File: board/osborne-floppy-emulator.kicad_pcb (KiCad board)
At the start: 2 copper layers, 61.6 x 54 mm, 82 parts, among them J1 Connector Out, J2 USB_A, J3 SWD Connector, J4 Connector In, Q1 BC557, Q2 BC547, Q3 T2N7002BK, Q4 BC847C, Q5 BC847C, Q6 BC847C, Q7 BC847C, Q8 BC847C, Q9 BC847C, U1 W25Q16JVSSIM, U2 RP2040, U3 TL494

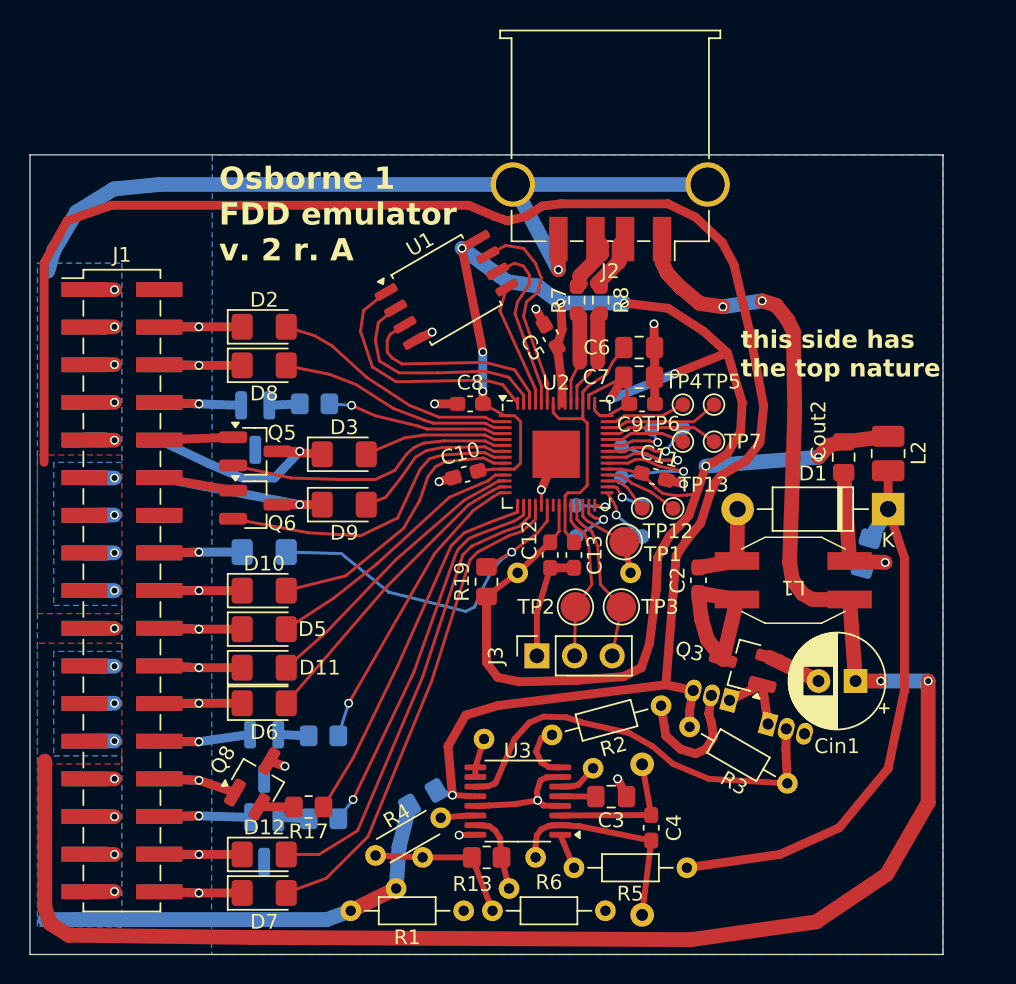
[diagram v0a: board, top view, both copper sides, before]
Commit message: shrink board slightly
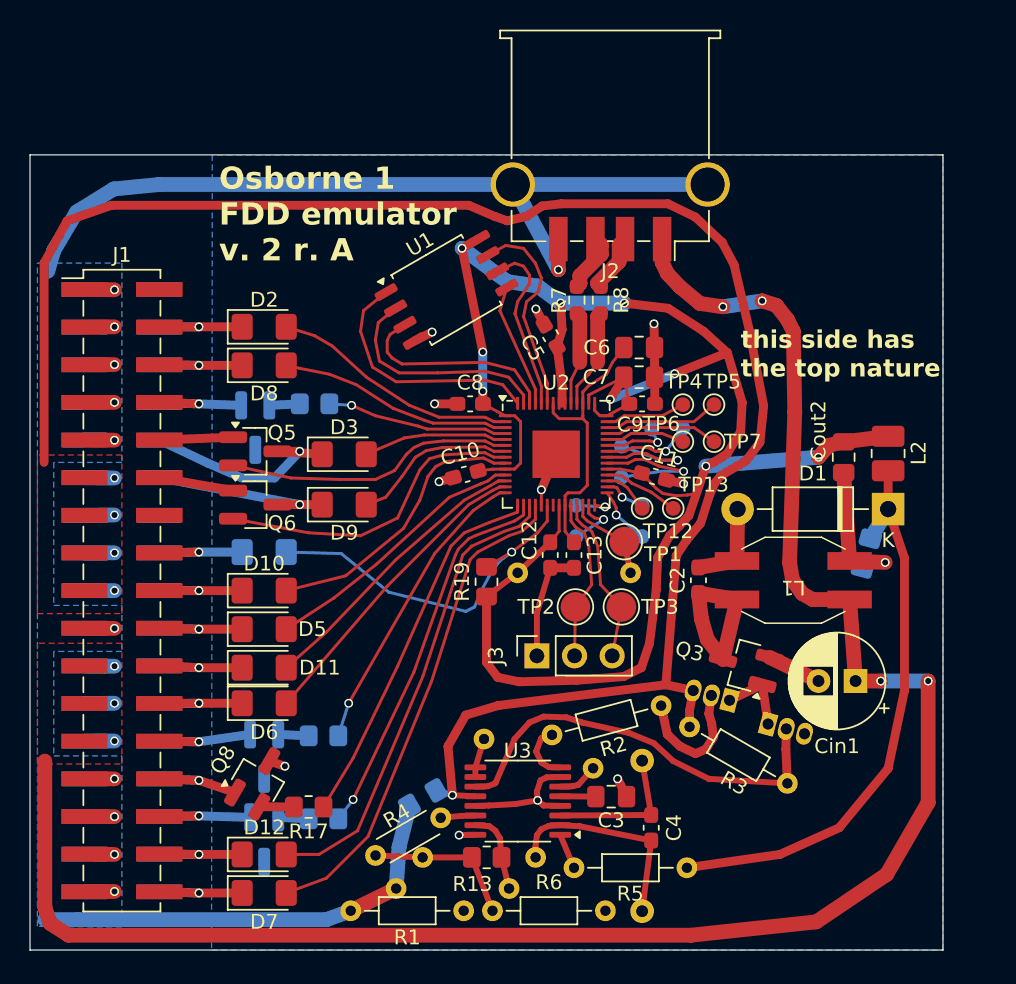
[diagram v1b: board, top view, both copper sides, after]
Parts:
- moved R11 0.25 mm to (131.7, 93.9)
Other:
- board size 61.6 x 54 mm -> 61.6 x 53.7 mm
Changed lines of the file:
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@@
 	(footprint "Resistor_THT:R_Axial_DIN0207_L6.3mm_D2.5mm_P10.16mm_Horizontal"
 		(layer "B.Cu")
-		(at 131.7 94.12 -90)
+		(at 131.7 93.87 -90)
 		(descr "Resistor, Axial_DIN0207 series, Axial, Horizontal, pin pitch=10.16mm, 0.25W = 1/4W, length*diameter=6.3*2.5mm^2, http://cdn-reichelt.de/documents/datenblatt/B400/1_4W%23YAG.pdf")
 		(tags "Resistor Axial_DIN0207 series Axial Horizontal pin pitch 10.16mm 0.25W = 1/4W length 6.3mm diameter 2.5mm")
@@
 	(gr_rect
 		(start 90.4 53)
-		(end 152 106.95)
+		(end 152 106.65)
 		(stroke
 			(width 0.05)
@@
 	)
 	(segment
-		(start 132.3125 99.2625)
-		(end 131.7 104.279999)
+		(start 126.175 98.225)
+		(end 125.4 98.275)
 		(width 0.4)
 		(layer "F.Cu")
@@
 	)
 	(segment
-		(start 126.175 98.225)
-		(end 125.4 98.275)
+		(start 127.5 98.3)
+		(end 132.3125 99.2625)
 		(width 0.4)
 		(layer "F.Cu")
@@
 	)
 	(segment
-		(start 127.5 98.3)
-		(end 132.3125 99.2625)
+		(start 132.3125 99.2625)
+		(end 131.7 104.03)
 		(width 0.4)
 		(layer "F.Cu")
@@
 	(segment
 		(start 132.3125 97.5375)
-		(end 131.7 94.12)
+		(end 131.7 93.87)
 		(width 0.4)
 		(layer "F.Cu")
@@
 	)
 	(segment
-		(start 91.4 103.75)
-		(end 91.4 93.9)
-		(width 1)
-		(layer "F.Cu")
-		(net 11)
-	)
-	(segment
-		(start 148.2 101.55)
-		(end 143.45 104.75)
+		(start 91.75 104.85)
+		(end 91.4 103.75)
 		(width 1)
 		(layer "F.Cu")
@@
 	)
 	(segment
-		(start 143.2 83)
-		(end 145.700001 83)
+		(start 91.4 103.75)
+		(end 91.4 93.9)
 		(width 1)
 		(layer "F.Cu")
@@
 	)
 	(segment
-		(start 151 88.5)
-		(end 151 96.7)
+		(start 143.2 83)
+		(end 145.700001 83)
 		(width 1)
 		(layer "F.Cu")
@@
 	)
 	(segment
-		(start 146.099999 88.5)
-		(end 147.8 88.5)
+		(start 151 96.7)
+		(end 148.2 101.55)
 		(width 1)
 		(layer "F.Cu")
@@
 	)
 	(segment
-		(start 91.75 104.85)
-		(end 91.4 103.75)
+		(start 148.2 101.55)
+		(end 143.45 104.75)
 		(width 1)
 		(layer "F.Cu")
@@
 	)
 	(segment
-		(start 135 105.95)
-		(end 105.4 105.8)
+		(start 146.099999 88.5)
+		(end 147.8 88.5)
 		(width 1)
 		(layer "F.Cu")
@@
 	)
 	(segment
-		(start 105.4 105.8)
-		(end 93 105.65)
+		(start 142.5 82.6)
+		(end 143.2 83)
 		(width 1)
 		(layer "F.Cu")
@@
 	)
 	(segment
-		(start 151 96.7)
-		(end 148.2 101.55)
+		(start 139.8 62.85)
+		(end 140.75 63.15)
 		(width 1)
 		(layer "F.Cu")
@@
 	)
 	(segment
-		(start 143.45 104.75)
-		(end 135 105.95)
+		(start 137.15 63.25)
+		(end 135.6 63.026923)
 		(width 1)
 		(layer "F.Cu")
@@
 	)
 	(segment
-		(start 142.5 82.6)
-		(end 143.2 83)
+		(start 141.9 64.9)
+		(end 142 70.35)
 		(width 1)
 		(layer "F.Cu")
@@
 	)
 	(segment
-		(start 93 105.65)
-		(end 91.75 104.85)
+		(start 141.5 64.1)
+		(end 141.9 64.9)
 		(width 1)
 		(layer "F.Cu")
@@
 	)
 	(segment
-		(start 139.8 62.85)
-		(end 140.75 63.15)
+		(start 93 105.65)
+		(end 91.75 104.85)
 		(width 1)
 		(layer "F.Cu")
@@
 	)
 	(segment
-		(start 137.15 63.25)
-		(end 135.6 63.026923)
+		(start 135 105.65)
+		(end 93 105.65)
 		(width 1)
 		(layer "F.Cu")
@@
 	)
 	(segment
-		(start 141.9 64.9)
-		(end 142 70.35)
+		(start 143.45 104.75)
+		(end 135 105.65)
 		(width 1)
 		(layer "F.Cu")
@@
 	)
 	(segment
-		(start 141.5 64.1)
-		(end 141.9 64.9)
+		(start 135.6 63.026923)
+		(end 134.25 61.9)
 		(width 1)
 		(layer "F.Cu")
@@
 	)
 	(segment
-		(start 135.6 63.026923)
-		(end 134.25 61.9)
+		(start 151 88.5)
+		(end 151 96.7)
 		(width 1)
 		(layer "F.Cu")
@@
 	)
 	(segment
-		(start 125.05 90.9)
-		(end 126.6 90.95)
-		(width 0.4)
-		(layer "F.Cu")
-		(net 50)
-	)
-	(segment
-		(start 126.6 90.95)
-		(end 127.65 91.3)
+		(start 121.3 95.6)
+		(end 121.8 95.4)
 		(width 0.4)
 		(layer "F.Cu")
@@
 	)
 	(segment
-		(start 136.2 95.1)
-		(end 141.499556 95.405)
+		(start 130.8 92)
+		(end 132.5 92.7)
 		(width 0.4)
 		(layer "F.Cu")
@@
 	)
 	(segment
-		(start 127.65 91.3)
-		(end 130.8 92)
+		(start 125.05 90.9)
+		(end 126.6 90.95)
 		(width 0.4)
 		(layer "F.Cu")
@@
 	)
 	(segment
-		(start 124.1 91.3)
-		(end 125.05 90.9)
+		(start 132.5 92.7)
+		(end 133.8 93.9)
 		(width 0.4)
 		(layer "F.Cu")
@@
 	)
 	(segment
-		(start 120.45 95.625)
-		(end 121.3 95.6)
+		(start 127.65 91.3)
+		(end 130.8 92)
 		(width 0.4)
 		(layer "F.Cu")
@@
 	)
 	(segment
-		(start 121.8 95.4)
-		(end 122.4 94)
+		(start 120.45 95.625)
+		(end 121.3 95.6)
 		(width 0.4)
 		(layer "F.Cu")
@@
 	)
 	(segment
-		(start 132.4 92.9)
-		(end 133.8 94.1)
+		(start 123.1 92.4)
+		(end 124.1 91.3)
 		(width 0.4)
 		(layer "F.Cu")
@@
 	)
 	(segment
-		(start 122.4 94)
-		(end 123.1 92.4)
+		(start 126.6 90.95)
+		(end 127.65 91.3)
 		(width 0.4)
 		(layer "F.Cu")
@@
 	)
 	(segment
-		(start 133.8 94.1)
-		(end 136.2 95.1)
+		(start 136.2 95.1)
+		(end 141.499556 95.405)
 		(width 0.4)
 		(layer "F.Cu")
@@
 	)
 	(segment
-		(start 121.3 95.6)
-		(end 121.8 95.4)
+		(start 121.8 95.4)
+		(end 122.4 94)
 		(width 0.4)
 		(layer "F.Cu")
@@
 	)
 	(segment
-		(start 130.8 92)
-		(end 132.4 92.9)
+		(start 122.4 94)
+		(end 123.1 92.4)
 		(width 0.4)
 		(layer "F.Cu")
@@
 	)
 	(segment
-		(start 123.1 92.4)
-		(end 124.1 91.3)
+		(start 133.8 93.9)
+		(end 136.2 95.1)
 		(width 0.4)
 		(layer "F.Cu")
@@
 	)
 	(segment
-		(start 136.4 91.4)
-		(end 136.2 90.7)
+		(start 124.1 91.3)
+		(end 125.05 90.9)
+		(width 0.4)
+		(layer "F.Cu")
+		(net 50)
+	)
+	(segment
+		(start 132.980178 90.1639)
+		(end 133.4 92.1)
 		(width 0.6)
 		(layer "F.Cu")
@@
 	)
 	(segment
-		(start 133.3 92.2)
-		(end 134.3 93.1)
+		(start 136 93.1)
+		(end 136.5 92.3)
 		(width 0.6)
 		(layer "F.Cu")
@@
 	)
 	(segment
-		(start 134.3 93.1)
-		(end 135.3 93.4)
+		(start 133.4 92.1)
+		(end 134.25 92.9)
 		(width 0.6)
 		(layer "F.Cu")
@@
 	)
 	(segment
-		(start 136.2 90.7)
-		(end 136.373273 89.4713)
+		(start 136.4 91.4)
+		(end 136.2 90.7)
 		(width 0.6)
 		(layer "F.Cu")
@@
 	)
 	(segment
-		(start 132.980178 90.1639)
-		(end 133.3 92.2)
+		(start 134.25 92.9)
+		(end 135.3 93.4)
 		(width 0.6)
 		(layer "F.Cu")
@@
 	)
 	(segment
-		(start 136 93.1)
-		(end 136.5 92.3)
+		(start 136.2 90.7)
+		(end 136.373273 89.4713)
 		(width 0.6)
 		(layer "F.Cu")
@@
 		(polygon
 			(pts
-				(xy 152 53) (xy 102.7 53) (xy 102.65 106.95) (xy 152 106.95)
+				(xy 152 53) (xy 102.7 53) (xy 102.65 106.65) (xy 152 106.65)
 			)
 		)
